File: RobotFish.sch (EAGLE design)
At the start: 14 parts, among them U1 MCP73831/OT, U3 MCP1754S_SOT23

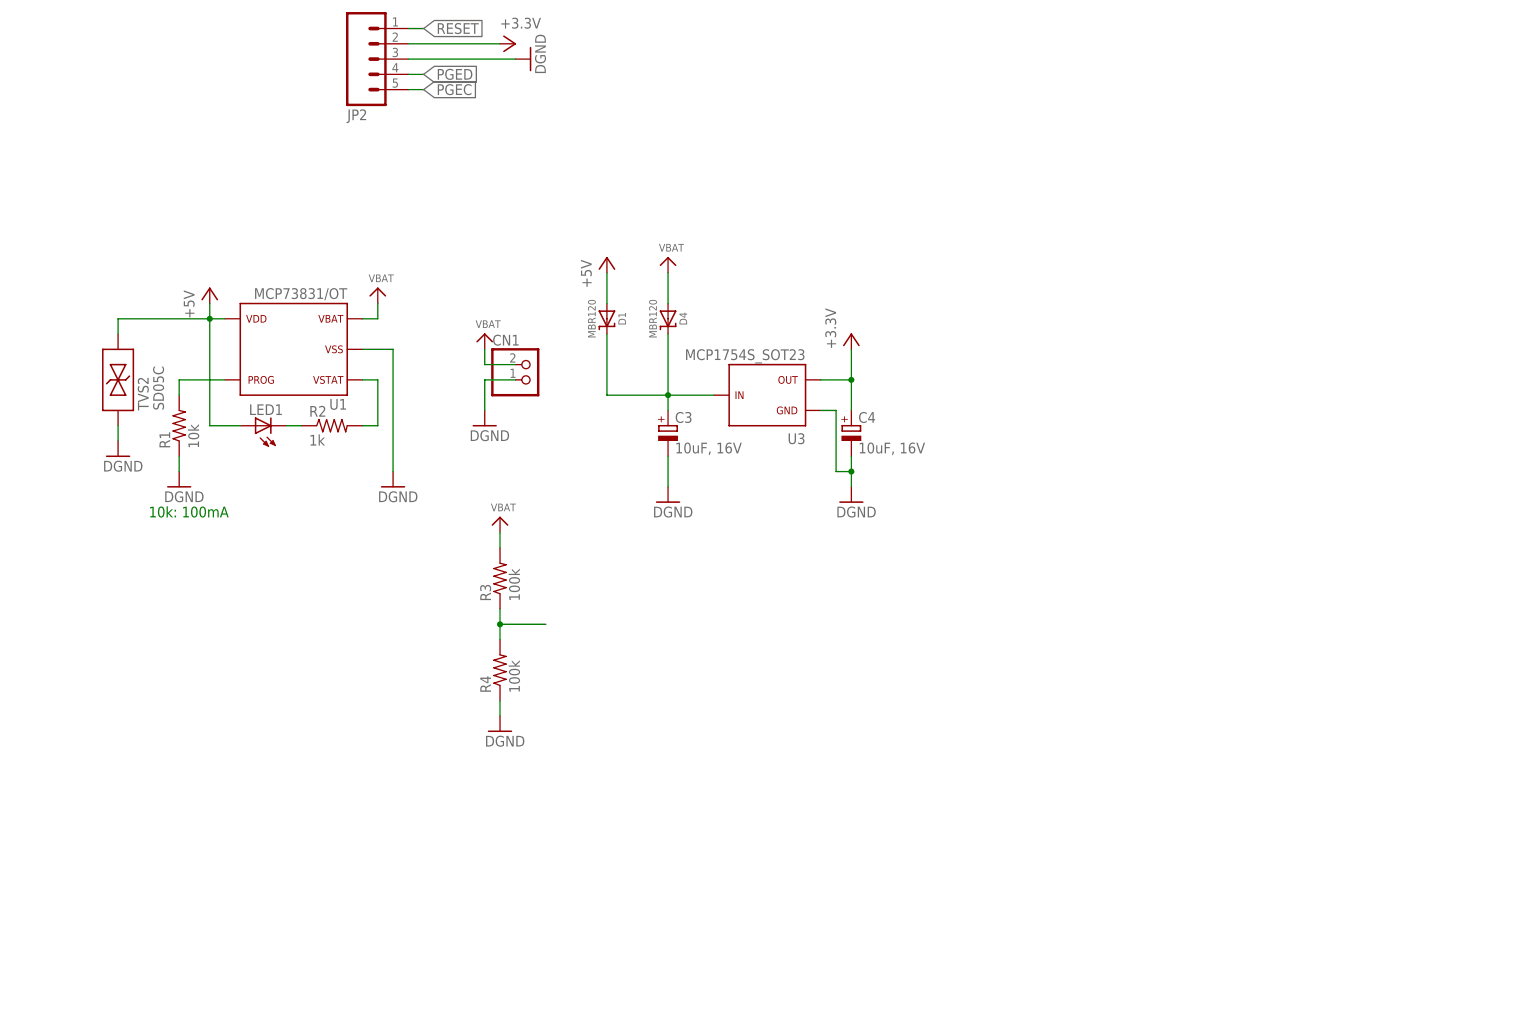
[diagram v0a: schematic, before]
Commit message: schematics
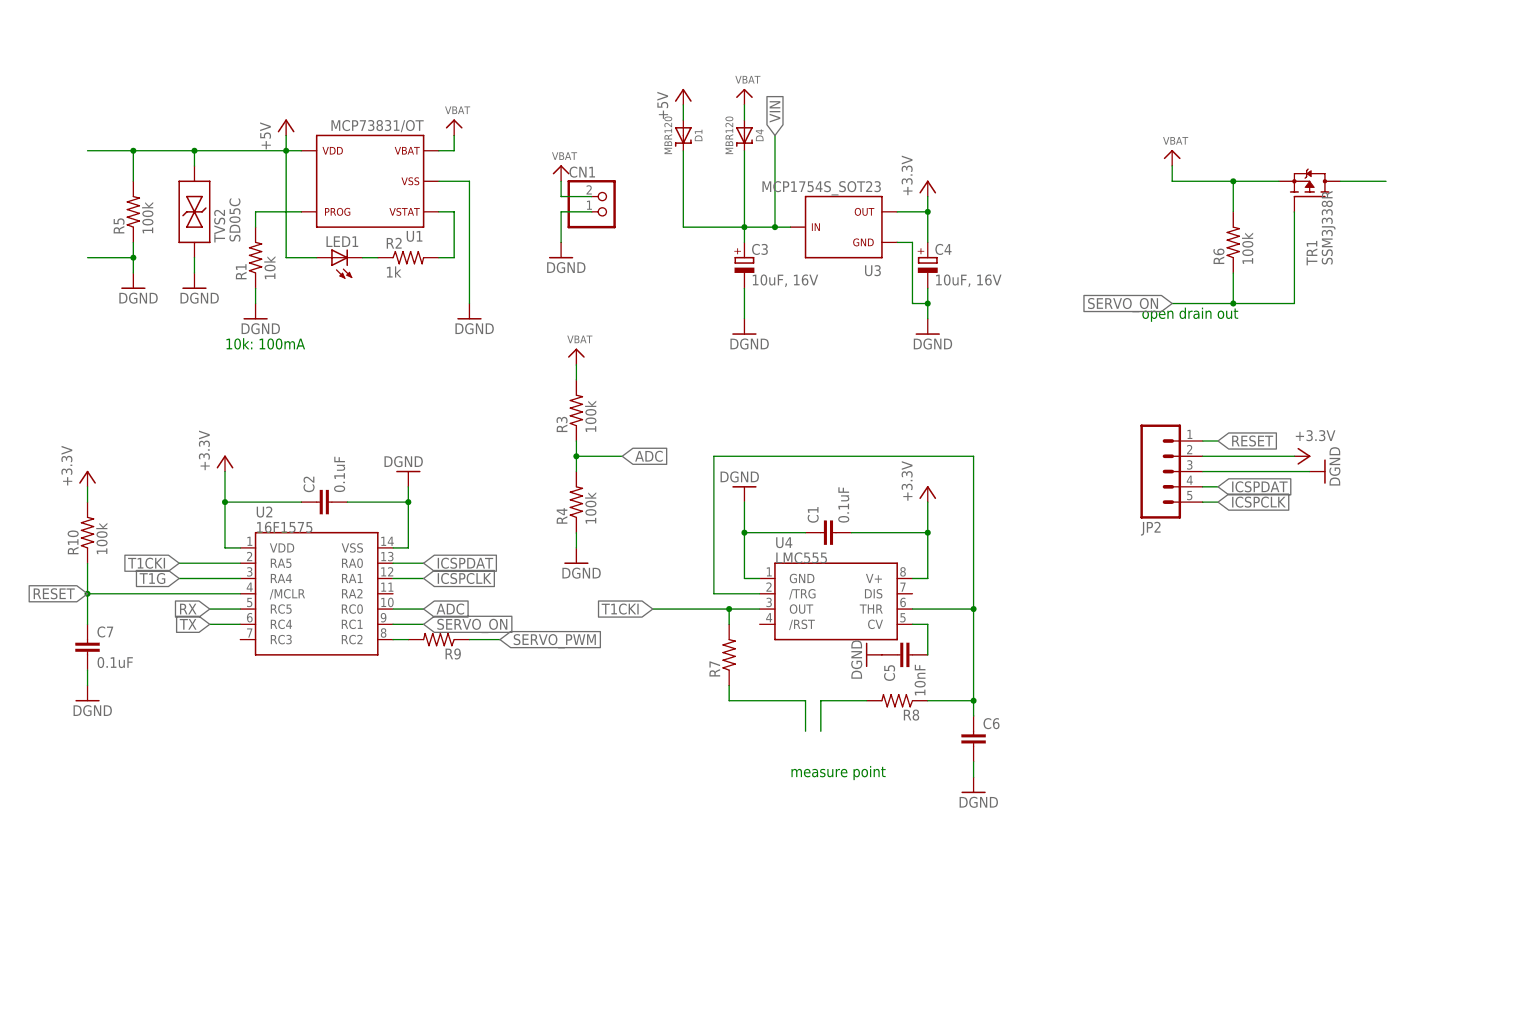
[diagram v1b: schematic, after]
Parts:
- added C1, C2, C7: 0.1uF, water:C0603(1608)
- added C5: 10nF, water:C0603(1608)
- added C6: (no value), water:C0805(2012)
- added R10, R5, R6: 100k, water:R0603(1608)
- added R7, R8, R9: (no value), water:R0603(1608)
- added TR1: SSM3J338R, water:SSM3J338R
- added U2: 16F1575, water:16F1575
- added U4: LMC555, water:LMC555
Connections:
- net N$5 renamed VIN
- removed net PGEC: JP2.5
- removed net PGED: JP2.4
- new net ADC: R3.1, R4.2, U2.RC0
- new net ICSPCLK: JP2.5, U2.RA1
- new net ICSPDAT: JP2.4, U2.RA0
- new net N$11: C5.2, U4.CV
- new net N$12: R7.1
- new net N$13: R8.2
- new net N$8: TR1.D
- new net N$9: C6.1, R8.1, U4./TRG, U4.THR
- new net RX: U2.RC5
- new net SERVO_ON: R6.1, TR1.G, U2.RC1
- new net SERVO_PWM: R9.1
- new net T1CKI: R7.2, U2.RA5, U4.OUT
- new net T1G: U2.RA4
- new net TX: U2.RC4
- net +3.3V: now also C1.2, C2.1, R10.2, U2.VDD, U4.V+
- net +5V: now also R5.2
- net DGND: now also C1.1, C2.2, C5.1, C6.2, C7.2, R5.1, U2.VSS, U4.GND
- net N$4: now also R9.2, U2.RC2; no longer R3.1, R4.2
- net RESET: now also C7.1, R10.1, U2./MCLR
- net VBAT: now also R6.2, TR1.S
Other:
- note added: "measure point"
- note added: "open drain out"
- moved on the sheet: C3, C4, CN1, D1, D4, JP2, LED1, R1, R2, R3, R4, TVS2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

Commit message: almost done
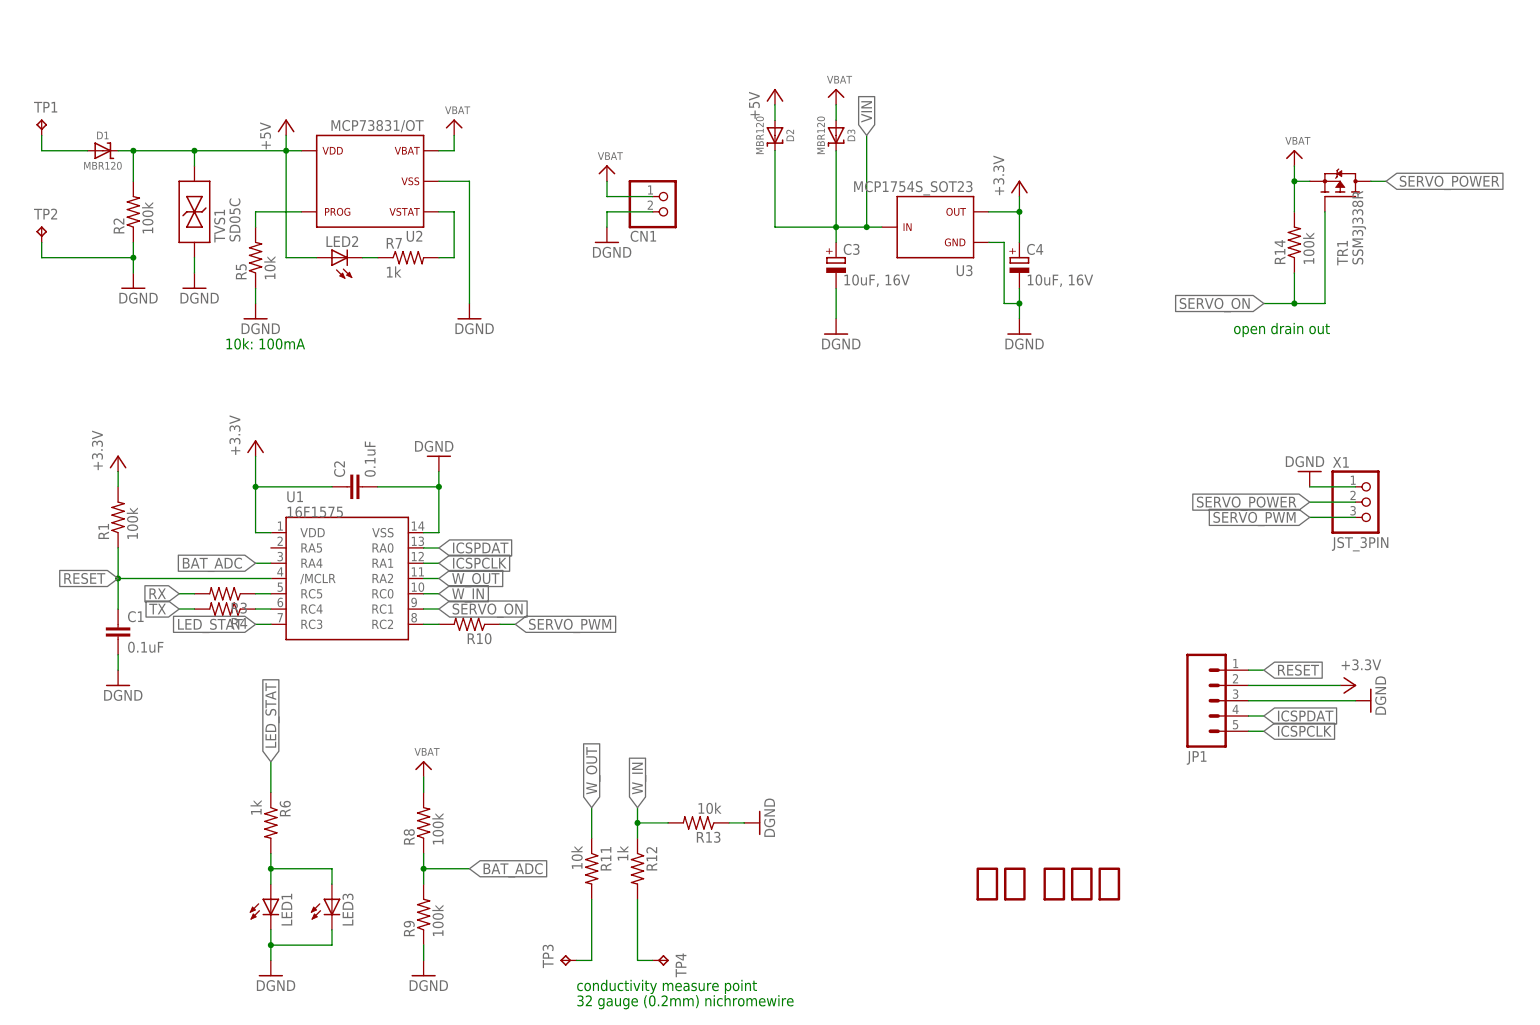
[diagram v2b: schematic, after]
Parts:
- removed C5: 10nF, water:C0603(1608)
- removed C6: (no value), water:C0805(2012)
- removed C7: 0.1uF, water:C0603(1608)
- removed D4: MBR120, microbuilder:DIODE-SCHOTTKYSOD-123
- removed JP2: (no value), SparkFun-Connectors:M05PTH
- removed U4: LMC555, water:LMC555
- added D2, D3: MBR120, microbuilder:DIODE-SCHOTTKYSOD-123
- added JP1: (no value), SparkFun-Connectors:M05PTH
- added LED2: (no value), berry:LED0603
- added LED3: (no value), berry:LED3MM
- added R11, R13: 10k, water:R0603(1608)
- added R12: 1k, water:R0603(1608)
- added R14: 100k, water:R0603(1608)
- added TP1, TP2, TP3, TP4: (no value), water:TP-5010
- added X1: JST_3PIN, water:JST_3PIN
- CN1: device adafruit:JST_2PIN-THM-RA -> water:JST_2PIN-THM-RA
- R1: value 10k -> 100k
- R10, R3, R4: value 100k -> (none)
- R2: value 1k -> 100k
- R5: value 100k -> 10k
- R6: value 100k -> 1k
- R7: value (none) -> 1k
- R8, R9: value (none) -> 100k
- U1: value MCP73831/OT -> 16F1575; device water:MCP73831/OT -> water:16F1575
- U2: value 16F1575 -> MCP73831/OT; device water:16F1575 -> water:MCP73831/OT
- renumbered TVS2 to TVS1
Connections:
- removed net ADC: R3.1, R4.2, U2.RC0
- removed net N$11: C5.2, U4.CV
- removed net N$12: R7.1
- removed net N$13: R8.2
- removed net N$9: C6.1, R8.1, U4./TRG, U4.THR
- removed net T1CKI: R7.2, U2.RA5, U4.OUT
- removed net T1G: U2.RA4
- new net BAT_ADC: R8.1, R9.2, U1.RA4
- new net LED_STAT: R6.1, U1.RC3
- new net N$15: R11.2, TP3.TP
- new net N$16: R12.2, TP4.TP
- new net N$5: D1.A, TP1.TP
- new net N$6: R3.1, U1.RC5
- new net N$7: R4.1, U1.RC4
- new net SERVO_POWER: TR1.D, X1.2
- new net W_IN: R12.1, R13.2, U1.RC0
- new net W_OUT: R11.1, U1.RA2
- net +3.3V: now also JP1.2, R1.2, U1.VDD; no longer C1.2, JP2.2, R10.2, U2.VDD, U4.V+
- net +5V: now also D1.C, D2.A, LED2.A, R2.2, U2.VDD; no longer D1.A, LED1.A, R5.2, U1.VDD
- net DGND: now also C1.2, CN1.1, JP1.3, LED1.C, LED3.C, R13.1, R2.1, R9.1, TP2.TP, X1.1; no longer C1.1, C5.1, C6.2, C7.2, CN1.2, JP2.3, R1.1, R4.1, U4.GND
- net ICSPCLK: now also JP1.5, U1.RA1; no longer JP2.5, U2.RA1
- net ICSPDAT: now also JP1.4, U1.RA0; no longer JP2.4, U2.RA0
- net N$1: now also R5.2, U2.PROG; no longer R1.2, U1.PROG
- net N$2: now also R7.2, U2.STAT; no longer R2.2, U1.STAT
- net N$3: now also LED2.C, R7.1; no longer LED1.C, R2.1
- net N$4: now also R10.2, U1.RC2; no longer R9.2, U2.RC2
- net N$8: now also LED1.A, LED3.A, R6.2; no longer TR1.D
- net RESET: now also C1.1, JP1.1, R1.1, U1./MCLR; no longer C7.1, JP2.1, R10.1, U2./MCLR
- net RX: now also R3.2; no longer U2.RC5
- net SERVO_ON: now also R14.1, U1.RC1; no longer R6.1, U2.RC1
- net SERVO_PWM: now also R10.1, X1.3; no longer R9.1
- net TX: now also R4.2; no longer U2.RC4
- net VBAT: now also CN1.2, D3.A, R14.2, R8.2, U2.VBAT; no longer CN1.1, D4.A, R3.2, R6.2, U1.VBAT
- net VIN: now also D2.C, D3.C; no longer D1.C, D4.C
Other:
- note added: "32 gauge (0.2mm) nichromewire"
- note added: "conductivity measure point"
- note added: "로봇 물고기"
- note removed: "measure point"
- moved on the sheet: C1, C2, C3, C4, CN1, D1, LED1, R1, R10, R2, R3, R4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

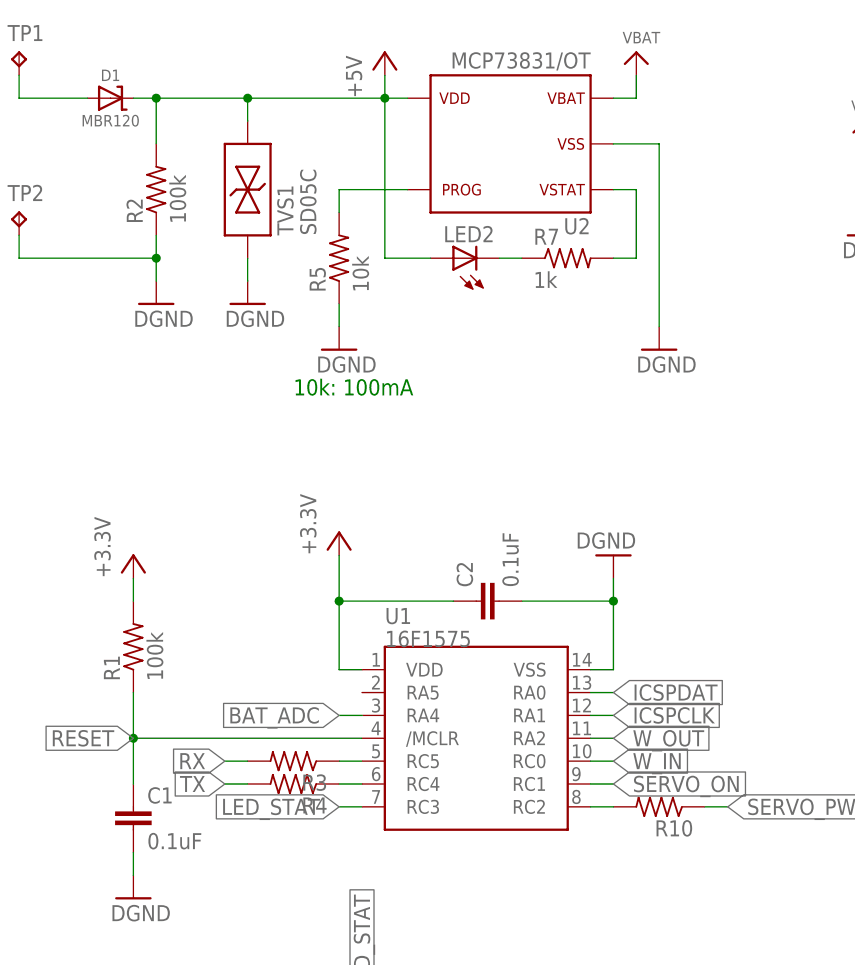
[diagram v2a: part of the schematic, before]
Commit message: value changed
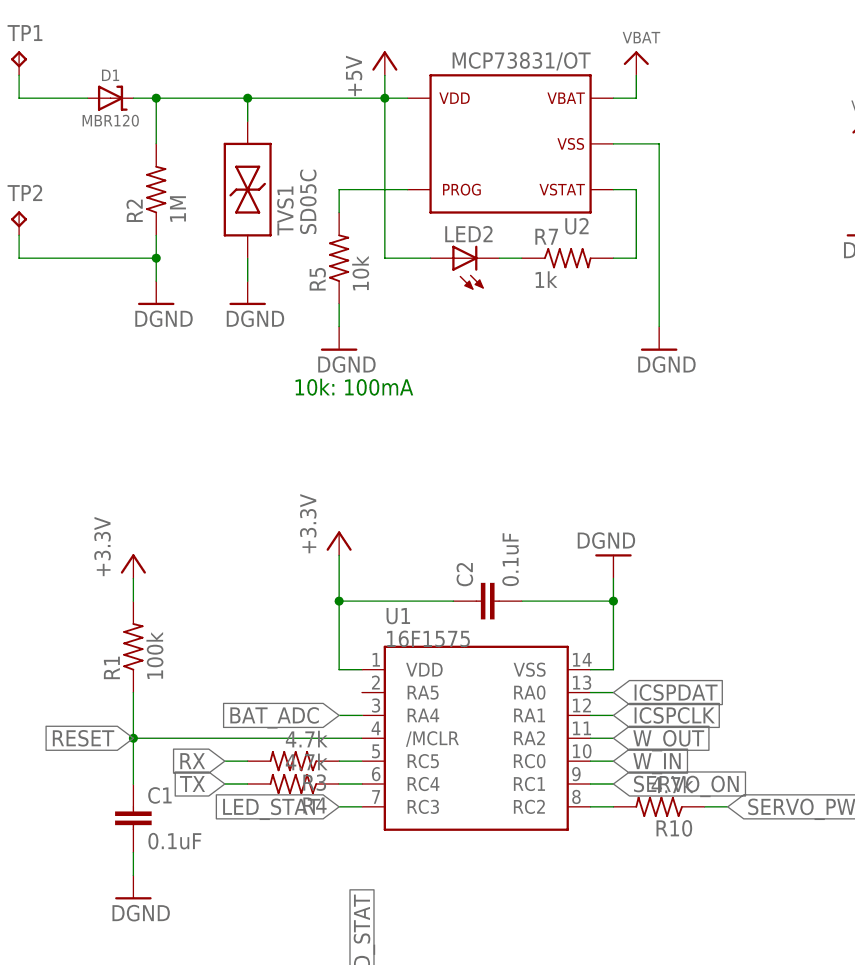
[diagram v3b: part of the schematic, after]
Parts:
- R10, R3, R4: value (none) -> 4.7k
- R2: value 100k -> 1M
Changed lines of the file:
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@@
 <part name="+3.3V1" library="berry" deviceset="+3.3V" device=""/>
 <part name="GND6" library="berry" deviceset="DGND" device=""/>
-<part name="R2" library="water" deviceset="R" device="0603(1608)" value="100k"/>
+<part name="R2" library="water" deviceset="R" device="0603(1608)" value="1M"/>
 <part name="GND7" library="berry" deviceset="DGND" device=""/>
 <part name="TR1" library="water" deviceset="SSM3J338R" device=""/>
 <part name="R14" library="water" deviceset="R" device="0603(1608)" value="100k"/>
 <part name="C2" library="water" deviceset="C" device="0603(1608)" value="0.1uF"/>
-<part name="R10" library="water" deviceset="R" device="0603(1608)"/>
+<part name="R10" library="water" deviceset="R" device="0603(1608)" value="4.7k"/>
 <part name="U$4" library="microbuilder" deviceset="VBAT" device=""/>
 <part name="R1" library="water" deviceset="R" device="0603(1608)" value="100k"/>
@@
 <part name="C1" library="water" deviceset="C" device="0603(1608)" value="0.1uF"/>
 <part name="D1" library="microbuilder" deviceset="DIODE-SCHOTTKY" device="SOD-123" value="MBR120"/>
-<part name="R3" library="water" deviceset="R" device="0603(1608)"/>
-<part name="R4" library="water" deviceset="R" device="0603(1608)"/>
+<part name="R3" library="water" deviceset="R" device="0603(1608)" value="4.7k"/>
+<part name="R4" library="water" deviceset="R" device="0603(1608)" value="4.7k"/>
 <part name="R6" library="water" deviceset="R" device="0603(1608)" value="1k"/>
 <part name="LED1" library="berry" deviceset="LED" device="0603"/>
